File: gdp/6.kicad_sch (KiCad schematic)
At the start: 1 part, among them U9 74LS83

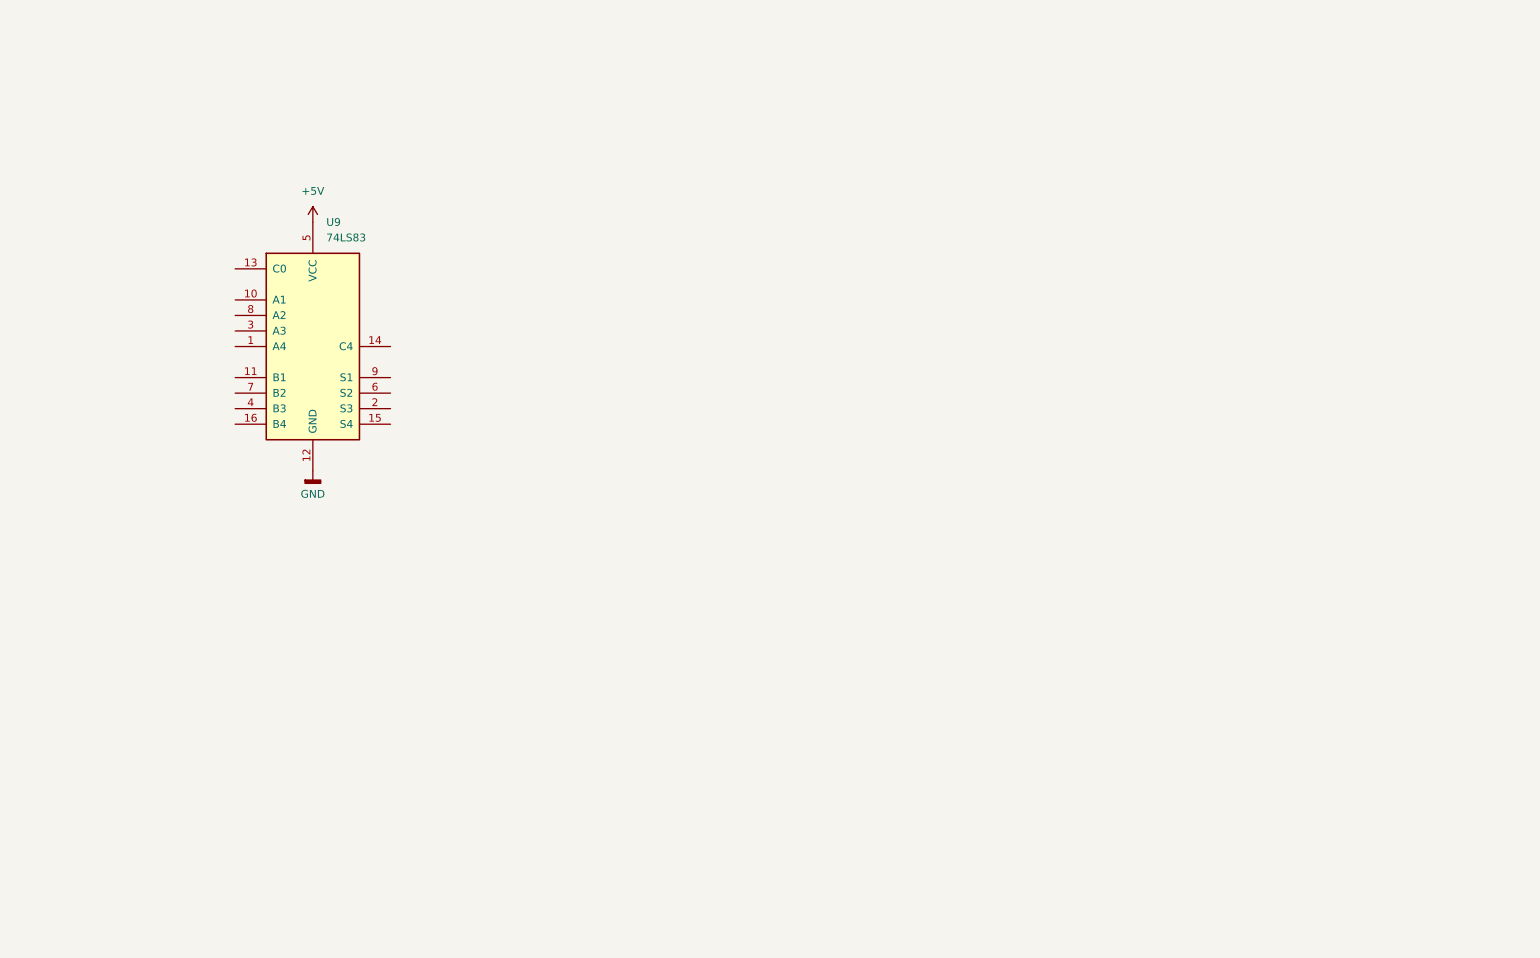
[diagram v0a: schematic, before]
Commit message: Adds Sheet 6
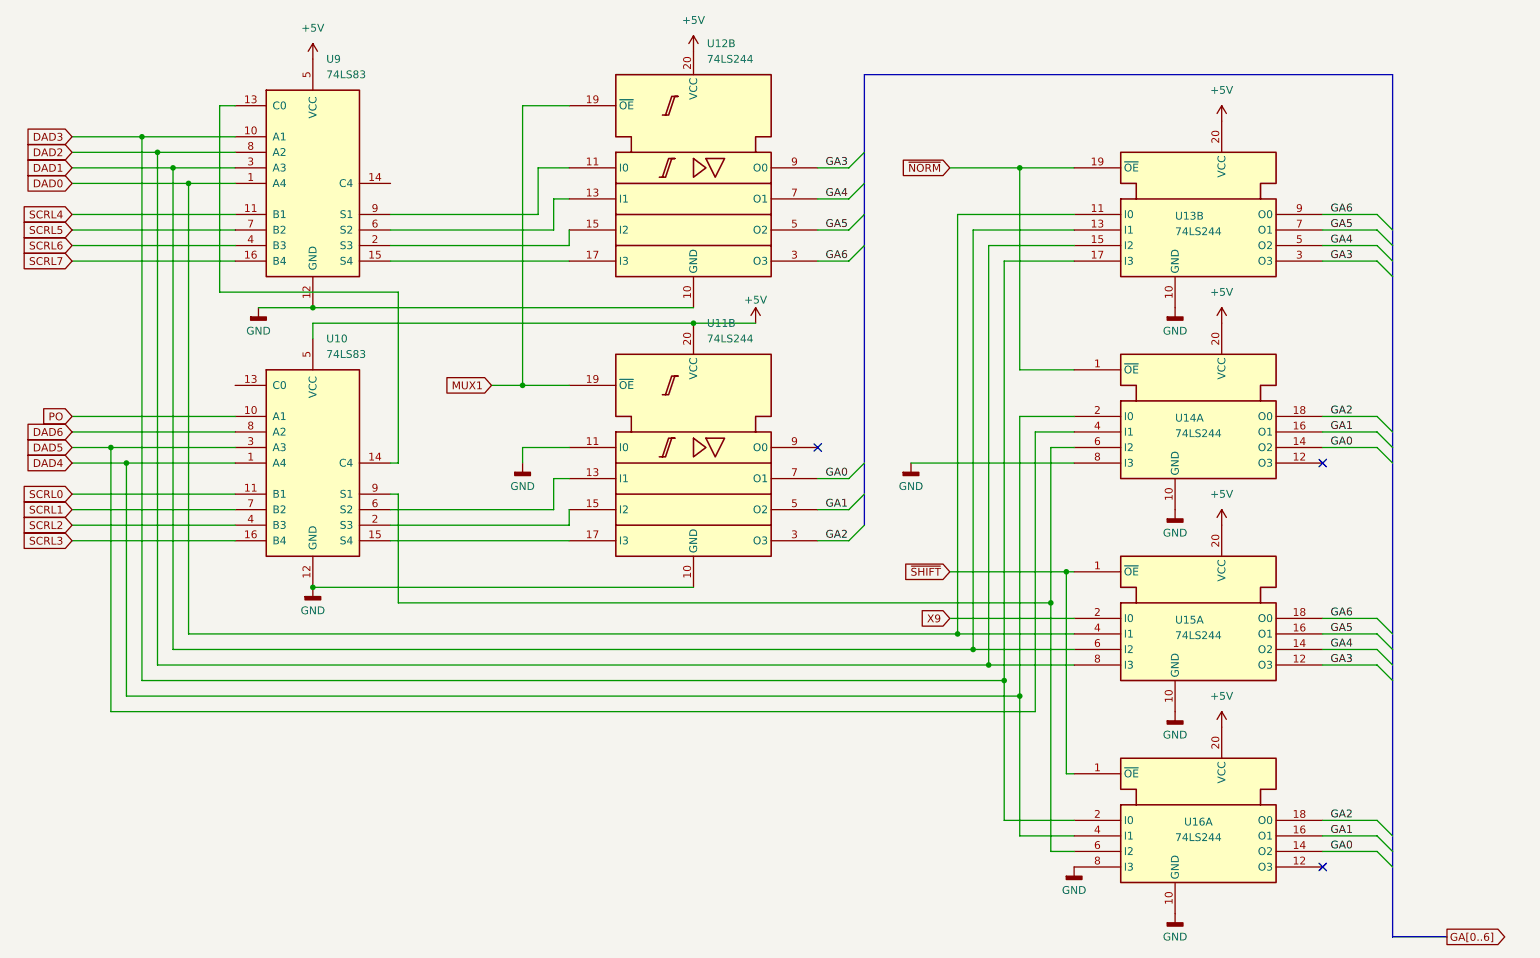
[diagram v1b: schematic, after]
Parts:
- added U10: 74LS83, symbol 74xx:74LS83
- added U11, U12, U13, U14, U15, U16: 74LS244, symbol 74xx_IEEE:74LS244
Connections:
- net +5V: now also U10.5 (VCC), U11.20 (VCC), U12.20 (VCC), U13.20 (VCC), U14.20 (VCC), U15.20 (VCC), U16.20 (VCC)
- net GND: now also U10.12 (GND), U11.10 (GND), U11.11 (I0), U12.10 (GND), U13.10 (GND), U14.10 (GND), U14.8 (I3), U15.10 (GND), U16.10 (GND), U16.8 (I3)
- net DAD0: now reaches U9.1 (A4)
- net DAD0: now also U13.11 (I0), U15.4 (I1)
- net DAD3: now reaches U9.10 (A1)
- net DAD3: now also U13.17 (I3), U16.2 (I0)
- net SCRL4: now reaches U9.11 (B1)
- net at U9.13 (C0): now also U10.14 (C4)
- net at U9.15 (S4): now also U12.17 (I3)
- net SCRL7: now reaches U9.16 (B4)
- net at U9.2 (S3): now also U12.15 (I2)
- net DAD1: now reaches U9.3 (A3)
- net DAD1: now also U13.13 (I1), U15.6 (I2)
- net SCRL6: now reaches U9.4 (B3)
- net at U9.6 (S2): now also U12.13 (I1)
- net SCRL5: now reaches U9.7 (B2)
- net DAD2: now reaches U9.8 (A2)
- net DAD2: now also U13.15 (I2), U15.8 (I3)
- net at U9.9 (S1): now also U12.11 (I0)
- new net: U10.6 (S2), U11.13 (I1)
- new net: U10.2 (S3), U11.15 (I2)
- new net: U10.15 (S4), U11.17 (I3)
- new net: U10.9 (S1), U14.6 (I2), U16.6 (I2)
- new net DAD4: U10.1 (A4), U14.2 (I0), U16.4 (I1)
- new net DAD5: U10.3 (A3), U14.4 (I1)
- new net DAD6: U10.8 (A2)
- new net GA0: U11.7 (O1), U14.14 (O2), U16.14 (O2)
- new net GA1: U11.5 (O2), U14.16 (O1), U16.16 (O1)
- new net GA2: U11.3 (O3), U14.18 (O0), U16.18 (O0)
- new net GA3: U12.9 (O0), U13.3 (O3), U15.12 (O3)
- new net GA4: U12.7 (O1), U13.5 (O2), U15.14 (O2)
- new net GA5: U12.5 (O2), U13.7 (O1), U15.16 (O1)
- new net GA6: U12.3 (O3), U13.9 (O0), U15.18 (O0)
- new net MUX1: U11.19 (~{OE}), U12.19 (~{OE})
- new net PO: U10.10 (A1)
- new net SCRL0: U10.11 (B1)
- new net SCRL1: U10.7 (B2)
- new net SCRL2: U10.4 (B3)
- new net SCRL3: U10.16 (B4)
- new net X9: U15.2 (I0)
- new net ~{NORM}: U13.19 (~{OE}), U14.1 (~{OE})
- new net ~{SHIFT}: U15.1 (~{OE}), U16.1 (~{OE})
- no-connect marks 0 -> 3
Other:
- moved on the sheet: U9
